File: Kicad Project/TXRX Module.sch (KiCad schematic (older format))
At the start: 19 parts, among them U10 GALI-2+, U11 BandpassFilter, U12 ufl, U13 Antenna111, U14 Antenna111, U15 ufl, U3 BandpassFilter, U9 LEE-39+

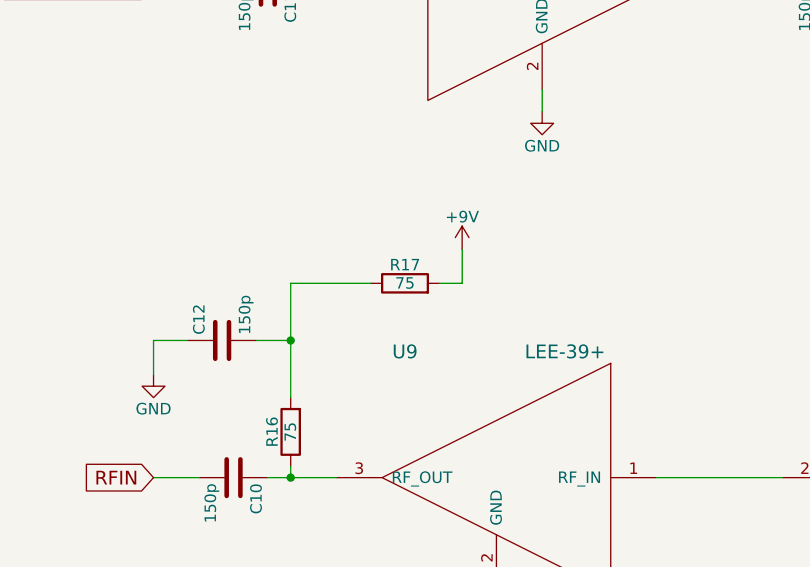
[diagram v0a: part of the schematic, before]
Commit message: PCB Pre Flood
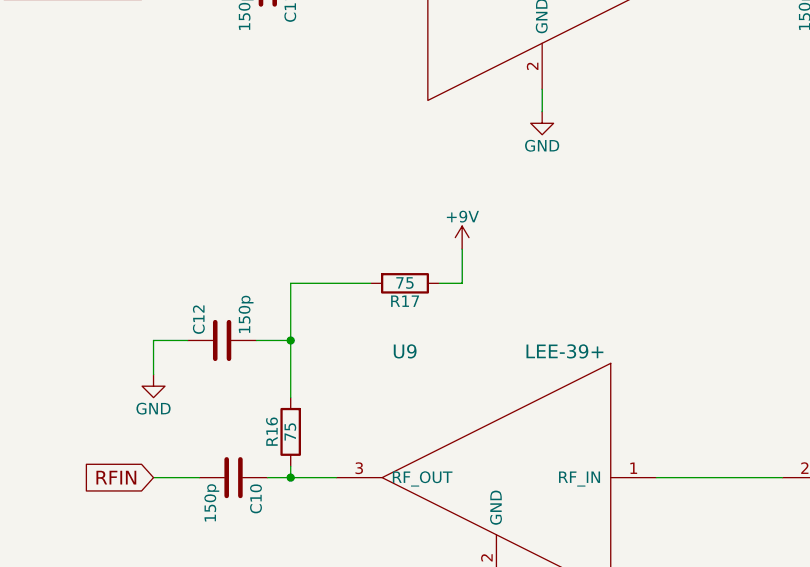
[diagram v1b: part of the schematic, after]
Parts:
- R17: footprint RadarComponents:100PAD -> RadarComponents:100PAD+GND
- R18: footprint RadarComponents:100PAD+GND -> RadarComponents:100PAD
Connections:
- net +9V: now also R17.1; no longer R17.2
- net at C12.2, R16.2: now also R17.2; no longer R17.1
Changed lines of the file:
@@
 F 0 "R18" V 5030 2450 50  0000 C CNN
 F 1 "75" V 4950 2450 50  0000 C CNN
-F 2 "RadarComponents:100PAD+GND" V 4880 2450 50  0001 C CNN
+F 2 "RadarComponents:100PAD" V 4880 2450 50  0001 C CNN
 F 3 "" H 4950 2450 50  0001 C CNN
 	1    4950 2450
@@
 F 0 "R17" V 3530 3950 50  0000 C CNN
 F 1 "75" V 3450 3950 50  0000 C CNN
-F 2 "RadarComponents:100PAD" V 3380 3950 50  0001 C CNN
+F 2 "RadarComponents:100PAD+GND" V 3380 3950 50  0001 C CNN
 F 3 "" H 3450 3950 50  0001 C CNN
 	1    3450 3950
-	0    -1   -1   0
+	0    1    1    0
 $EndComp
 $Comp
